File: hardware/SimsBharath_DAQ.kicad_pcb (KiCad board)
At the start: 2 copper layers, 74.5 x 119.5 mm, 108 parts, among them J1 Conn_02x05_Odd_Even, J10 702471052, J11 702471052, J2 USB1030-GF-P-B-B, J3 702471052, J4 702471052, J5 702471052, J6 702471052, J7 702471052, J8 702471052, J9 1-406507-5, SW1 SW_Push, U1 STM32H753ZIT6, U2 MIC37100-3.3WS, U3 LAN8742A-CZ-TR, U4 H1102NL, X1 XRCGB25M000F3A16R0, X2 XRCGB25M000F3A16R0, X3 CM7V-T1A-32.768KHZ-7PF-20PPM-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

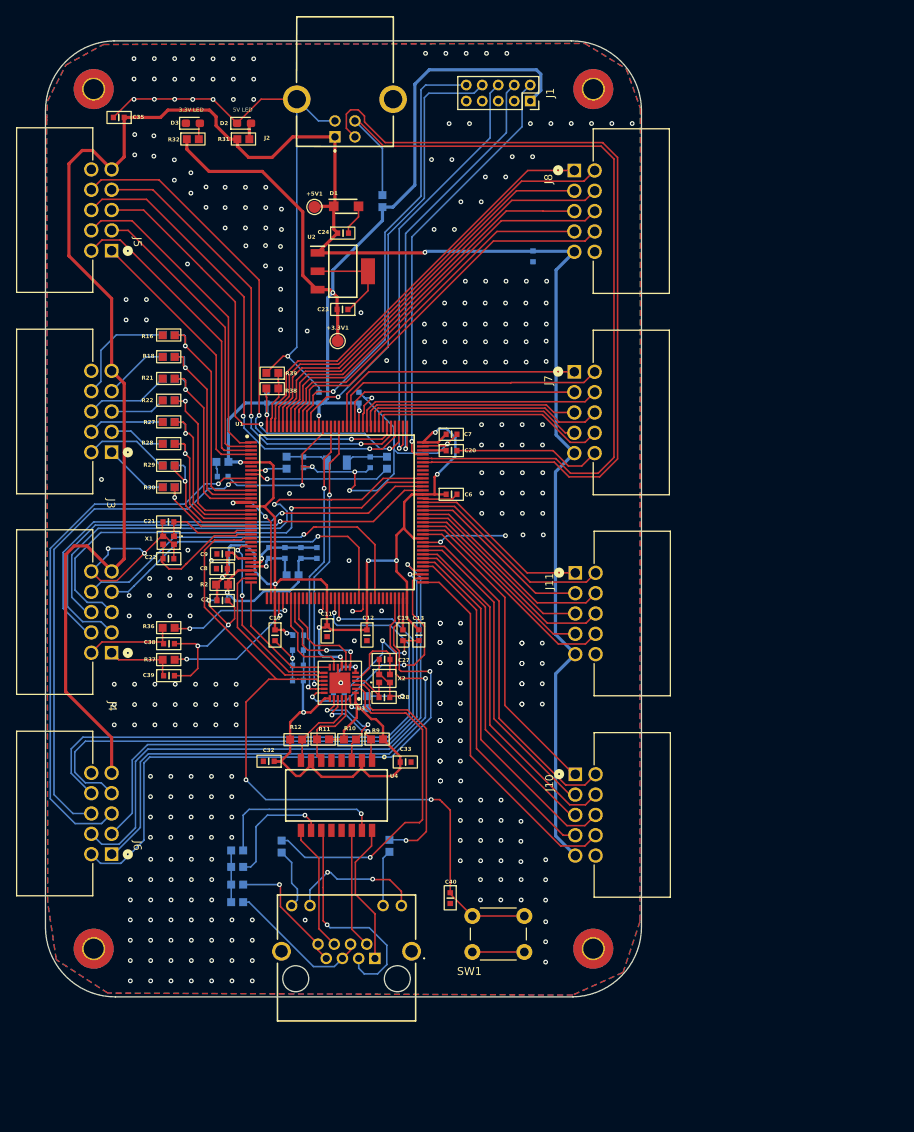
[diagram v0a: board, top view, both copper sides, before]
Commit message: completed the design with perfect mechanics
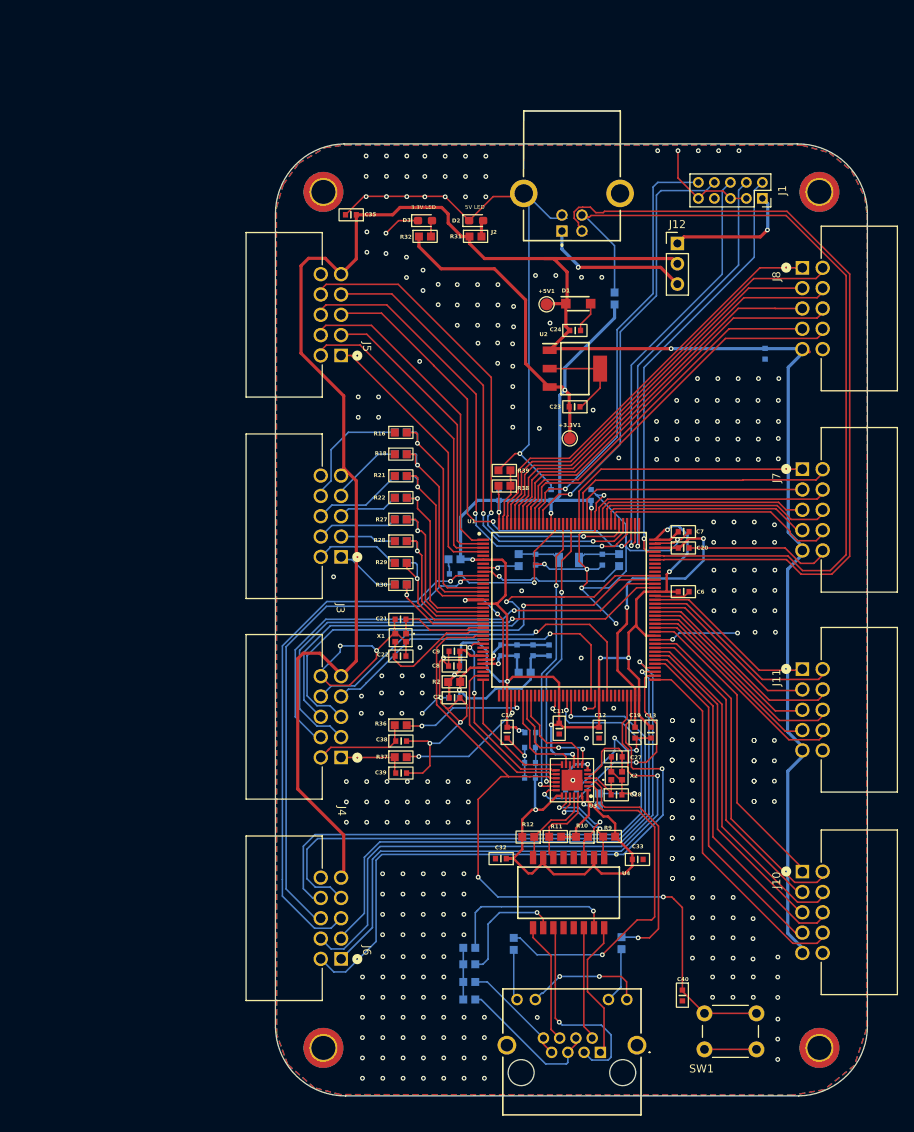
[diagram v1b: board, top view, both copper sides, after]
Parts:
- removed the REF** at (133.7, 30.7)
- removed the REF** at (133.7, 138.1)
- removed the REF** at (71.3, 138.1)
- removed the REF** at (71.3, 30.7)
- added J12: Conn_01x03, Connector_PinHeader_2.54mm:PinHeader_1x03_P2.54mm_Vertical, F.Cu at (144.2, 50.0)
- added REF**: MountingHole_2.5mm_Pad_TopBottom, MountingHole:MountingHole_2.5mm_Pad_TopBottom, F.Cu at (162.0, 150.5)
- added REF**: MountingHole_2.5mm_Pad_TopBottom, MountingHole:MountingHole_2.5mm_Pad_TopBottom, F.Cu at (100.0, 43.5)
- added REF**: MountingHole_2.5mm_Pad_TopBottom, MountingHole:MountingHole_2.5mm_Pad_TopBottom, F.Cu at (100.0, 150.5)
- added REF**: MountingHole_2.5mm_Pad_TopBottom, MountingHole:MountingHole_2.5mm_Pad_TopBottom, F.Cu at (162.0, 43.5)
- moved J3 31.5 mm to (102.2, 89.2)
- moved J4 31.5 mm to (102.2, 114.2)
- moved J5 31.5 mm to (102.2, 64.0)
- moved J6 31.5 mm to (102.2, 139.4)
- moved C11 31.5 mm to (129.5, 110.6)
- moved C25 31.5 mm to (130.9, 118.3)
- moved C6 31.5 mm to (145.0, 93.5)
- moved C7 31.5 mm to (145.0, 86.0)
- moved C8 31.5 mm to (116.3, 102.8)
- moved D3 31.5 mm to (112.7, 47.1)
- moved U3 31.5 mm to (131.1, 117.1)
- moved C1 31.5 mm to (116.3, 106.8)
- moved C20 31.5 mm to (145.0, 88.0)
- moved C24 31.5 mm to (131.5, 60.8)
- moved R4 31.5 mm to (134.4, 119.5)
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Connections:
- J1 pad 1: +3.3V -> /CONNECTORS/+5V-JTAG
- J2 pad 1: +5V -> /CONNECTORS/+5V-USB
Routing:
- net GND: track 335.3 -> 382.2 mm, vias 328 -> 316
- net +3.3V: track 274.7 -> 236.3 mm
- net VCAP: track 6.88 -> 39.4 mm, vias 0 -> 2
- net /CONNECTORS/+5V-USB: track 0.00 -> 18.6 mm, vias 0 -> 1
- net /CONNECTORS/+5V-JTAG: track 0.00 -> 16.2 mm, vias 0 -> 1
- net +5V: track 269.7 -> 282.5 mm
- net Net-(J9-Pad7): track 16.4 -> 13.6 mm, vias 1 -> 0
- net /CONNECTORS/RX P: track 28.6 -> 26.0 mm
- net /CONNECTORS/UART1_RX: track 75.4 -> 76.8 mm
- net Net-(J9-A_GREEN_2): track 7.75 -> 6.37 mm
- net /CONNECTORS/I2C2_SCL: track 73.1 -> 74.4 mm
- net /CONNECTORS/USB_FS_D P: track 108.0 -> 106.7 mm
- net /CONNECTORS/UART2_TX: track 67.9 -> 69.0 mm
- net /CONNECTORS/ADC3_2: track 8.15 -> 9.22 mm
- net /CONNECTORS/ADC3_1: track 14.1 -> 15.2 mm
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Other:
- board size 74.5 x 119.5 mm -> 74 x 119 mm
